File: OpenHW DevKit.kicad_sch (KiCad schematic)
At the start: 87 parts, among them Q1 MMBT3904, Q2 MMBT3904, Q3 MMBT3904, Q4 MMBT3904, SW1 SW_Push, SW2 SW_Push, U10 PI4ULS3V302XVEX, U13 PI4ULS3V302XVEX, U14 CORE-V-MCU, U15 PI4ULS3V302XVEX, U16 PI4ULS3V302XVEX, U17 PI4ULS3V302XVEX, U18 PI4ULS3V302XVEX, U19 PI4ULS3V302XVEX, U3 W25Q32JWZP, U4 PI6ULS5V9306WEX, U5 MAX6842DUKD0+T, U6 PI4ULS3V302XVEX, U7 PI4ULS3V302XVEX, U8 PI4ULS3V302XVEX, U9 PI4ULS3V302XVEX, X1 ECS-2520MVLC-100-CN

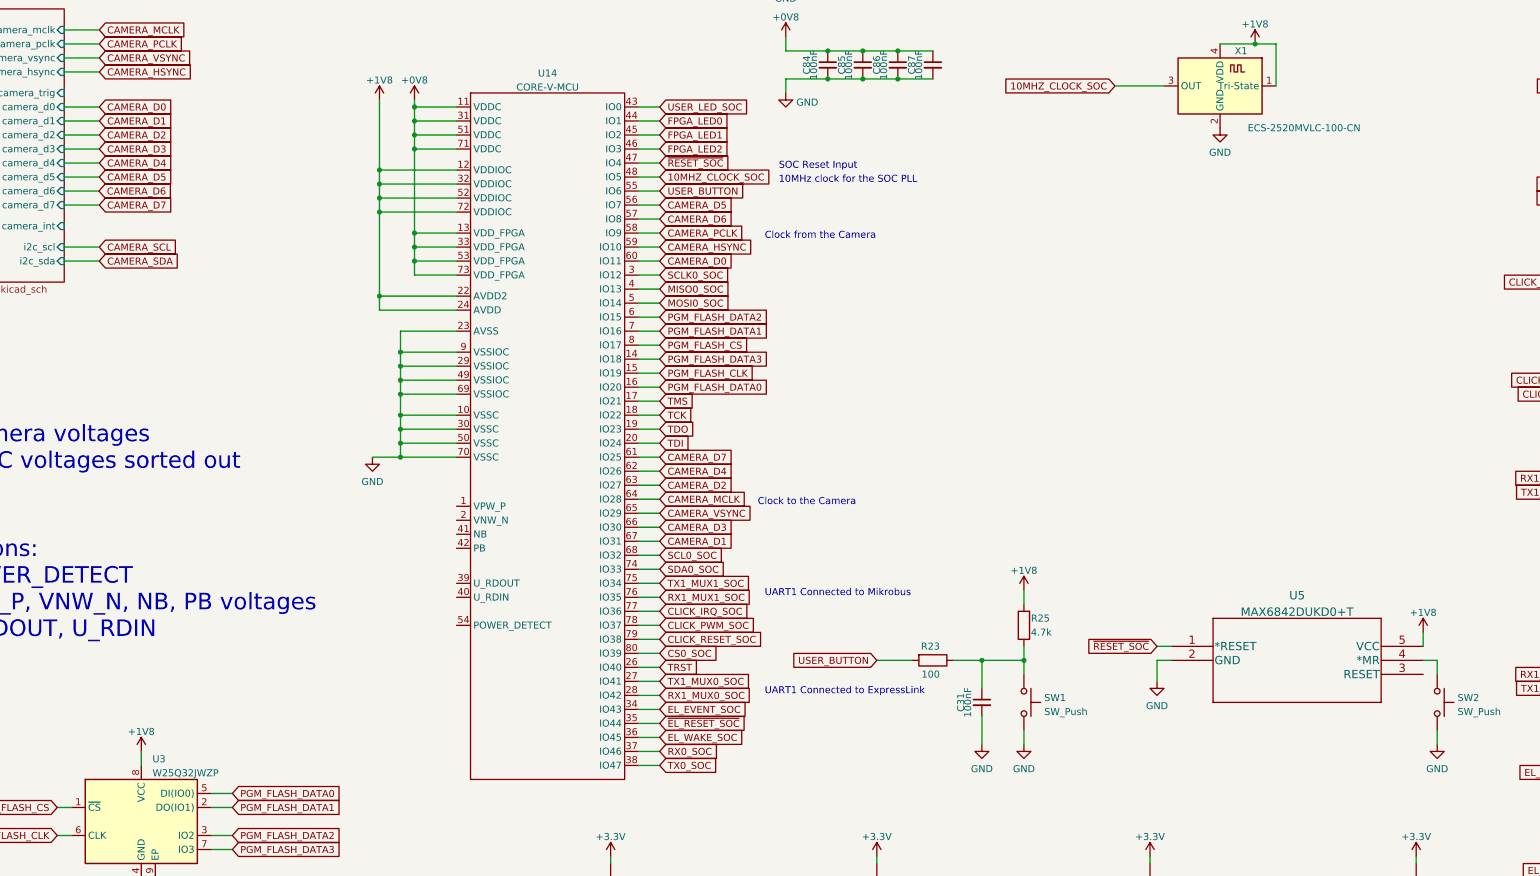
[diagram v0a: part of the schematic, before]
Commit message: revised pinout
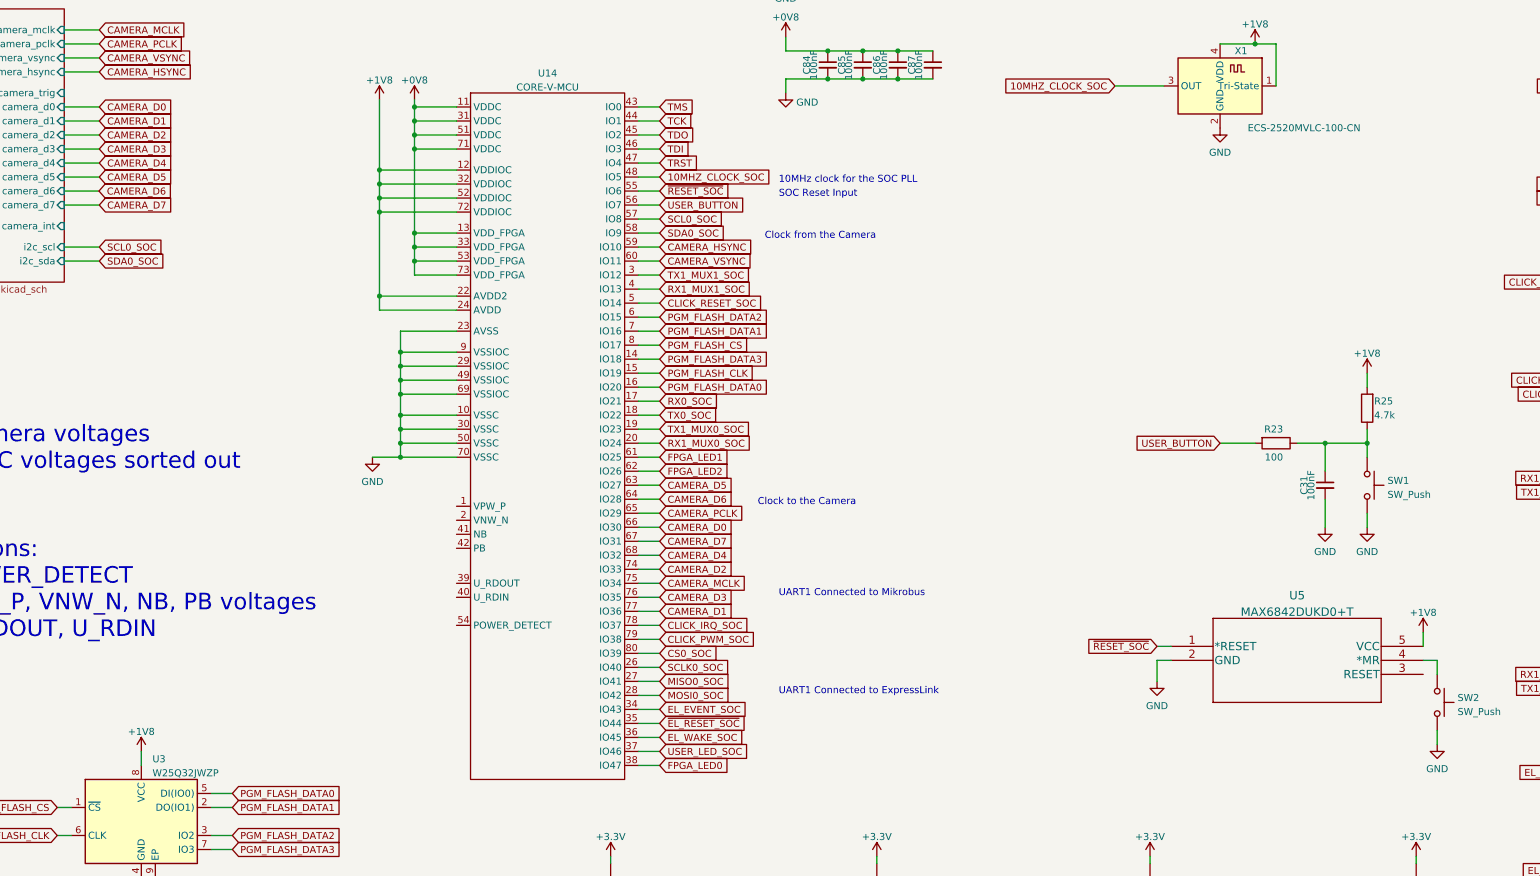
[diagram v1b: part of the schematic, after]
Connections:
- net CAMERA_D0: now also U14.66 (IO30); no longer U14.60 (IO11)
- net CAMERA_D1: now also U14.77 (IO36); no longer U14.67 (IO31)
- net CAMERA_D2: now also U14.74 (IO33); no longer U14.63 (IO27)
- net CAMERA_D3: now also U14.76 (IO35); no longer U14.66 (IO30)
- net CAMERA_D4: now also U14.68 (IO32); no longer U14.62 (IO26)
- net CAMERA_D5: now also U14.63 (IO27); no longer U14.56 (IO7)
- net CAMERA_D6: now also U14.64 (IO28); no longer U14.57 (IO8)
- net CAMERA_D7: now also U14.67 (IO31); no longer U14.61 (IO25)
- net CAMERA_MCLK: now also U14.75 (IO34); no longer U14.64 (IO28)
- net CAMERA_PCLK: now also U14.65 (IO29); no longer U14.58 (IO9)
- net CAMERA_VSYNC: now also U14.60 (IO11); no longer U14.65 (IO29)
- net CLICK_IRQ_SOC: now also U14.78 (IO37); no longer U14.77 (IO36)
- net CLICK_PWM_SOC: now also U14.79 (IO38); no longer U14.78 (IO37)
- net CLICK_RESET_SOC: now also U14.5 (IO14); no longer U14.79 (IO38)
- net FPGA_LED0: now also U14.38 (IO47); no longer U14.44 (IO1)
- net FPGA_LED1: now also U14.61 (IO25); no longer U14.45 (IO2)
- net FPGA_LED2: now also U14.62 (IO26); no longer U14.46 (IO3)
- net MISO0_SOC: now also U14.27 (IO41); no longer U14.4 (IO13)
- net MOSI0_SOC: now also U14.28 (IO42); no longer U14.5 (IO14)
- net RX0_SOC: now also U14.17 (IO21); no longer U14.37 (IO46)
- net RX1_MUX0_SOC: now also U14.20 (IO24); no longer U14.28 (IO42)
- net RX1_MUX1_SOC: now also U14.4 (IO13); no longer U14.76 (IO35)
- net SCL0_SOC: now also U14.57 (IO8); no longer U14.68 (IO32)
- net SCLK0_SOC: now also U14.26 (IO40); no longer U14.3 (IO12)
- net SDA0_SOC: now also U14.58 (IO9); no longer U14.74 (IO33)
- net TCK: now also U14.44 (IO1); no longer U14.18 (IO22)
- net TDI: now also U14.46 (IO3); no longer U14.20 (IO24)
- net TDO: now also U14.45 (IO2); no longer U14.19 (IO23)
- net TMS: now also U14.43 (IO0); no longer U14.17 (IO21)
- net TRST: now also U14.47 (IO4); no longer U14.26 (IO40)
- net TX0_SOC: now also U14.18 (IO22); no longer U14.38 (IO47)
- net TX1_MUX0_SOC: now also U14.19 (IO23); no longer U14.27 (IO41)
- net TX1_MUX1_SOC: now also U14.3 (IO12); no longer U14.75 (IO34)
- net USER_BUTTON: now also U14.56 (IO7); no longer U14.55 (IO6)
- net USER_LED_SOC: now also U14.37 (IO46); no longer U14.43 (IO0)
- net ~{RESET_SOC}: now also U14.55 (IO6); no longer U14.47 (IO4)
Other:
- moved on the sheet: C31, R23, R25, SW1

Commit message: Changed to KiCAD 7 and updated to final pinout.
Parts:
- removed C26, C27, C30, C38, C39, C42, C43, C44, C46, C47, C52, C53, C54, C56, C58, C60, C62, C64, C66, C67: 100nF, Capacitor_SMD:C_0603_1608Metric, symbol Device:C_Small
- removed U10, U13, U15, U16, U17, U18, U19, U6, U7, U8, U9: PI4ULS3V302XVEX, pi4uls3v302:PSON40P160X120X55-8N, symbol PI4ULS3V302XVEX:PI4ULS3V302XVEX
- removed U4: PI6ULS5V9306WEX, Package_SO:SOIC-8_3.9x4.9mm_P1.27mm, symbol PI6ULS5V9306:PI6ULS5V9306WEX
- added J10, J7, J8, J9: Conn_01x20, Connector_PinHeader_1.00mm:PinHeader_1x20_P1.00mm_Vertical, symbol Connector_Generic:Conn_01x20
- added JP2, JP6, JP7, JP8: SolderJumper_2_Bridged, Jumper:SolderJumper-2_P1.3mm_Bridged_RoundedPad1.0x1.5mm, symbol Jumper:SolderJumper_2_Bridged
- added SYM*1: ~, logos:devkits_qr, symbol OpenHW:Devkit_QR
- added TP1: TestPoint, TestPoint:TestPoint_Pad_D1.0mm, symbol Connector:TestPoint
- added U4: FXMA2102UMX, FXMA2102UMX:FXMA2102UMX, symbol FXMA2102UMX:FXMA2102UMX
- added U6, U7, U8, U9: NTB0104BQ,115, NTB0104:NXP_Semiconductors-SOT762-1-08_2019-0-MFG, symbol NTB0104:NTB0104BQ,115
- SW1, SW2: footprint Button_Switch_SMD:SW_Push_1P1T-SH_NO_CK_KMR2xxG -> Button:TS204225WT160SMTTR
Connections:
- net +0V8: now also U14.35 (VDD_FPGA), J10.11 (Pin_11), J10.13 (Pin_13), J7.11 (Pin_11), J7.13 (Pin_13), J8.13 (Pin_13), J8.15 (Pin_15), J9.11 (Pin_11), J9.13 (Pin_13); no longer U14.31 (VDDC)
- net +1V8: now also U14.23 (AVDD2), U14.25 (AVDD), U14.34 (VDDIOC), J10.12 (Pin_12), J7.12 (Pin_12), J8.14 (Pin_14), J8.3 (Pin_3), J8.5 (Pin_5), J9.12 (Pin_12), JP2.1 (A), JP8.1 (A), U4.8 (VCCB), U6.1 (VCC(A)), U6.8 (OE), U7.1 (VCC(A)), U7.8 (OE), U8.1 (VCC(A)), U8.8 (OE), U9.1 (VCC(A)), U9.8 (OE); no longer U14.22 (AVDD2), U14.24 (AVDD), U14.32 (VDDIOC)
- net +3V3: now also U6.14 (VCC(B)), U7.14 (VCC(B)), U8.14 (VCC(B)), U9.14 (VCC(B))
- net 10MHZ_CLOCK_SOC: now also J9.8 (Pin_8)
- net CAMERA_D0: now also U14.77 (IO30), J10.17 (Pin_17); no longer U14.66 (IO30)
- net CAMERA_D1: now also U14.67 (IO36), J10.7 (Pin_7); no longer U14.77 (IO36)
- net CAMERA_D2: now also U14.68 (IO33), J10.8 (Pin_8); no longer U14.74 (IO33)
- net CAMERA_D3: now also U14.64 (IO35), J10.4 (Pin_4); no longer U14.76 (IO35)
- net CAMERA_D4: now also U14.76 (IO32), J10.16 (Pin_16); no longer U14.68 (IO32)
- net CAMERA_D5: now also U14.36 (IO27), J8.16 (Pin_16); no longer U14.63 (IO27)
- net CAMERA_D6: now also U14.78 (IO28), J10.18 (Pin_18); no longer U14.64 (IO28)
- net CAMERA_D7: now also U14.74 (IO31), J10.14 (Pin_14); no longer U14.67 (IO31)
- net CAMERA_HSYNC: now also U14.20 (IO10), J7.20 (Pin_20); no longer U14.59 (IO10)
- net CAMERA_MCLK: now also U14.63 (IO34), J10.3 (Pin_3); no longer U14.75 (IO34)
- net CAMERA_PCLK: now also U14.66 (IO29), J10.6 (Pin_6); no longer U14.65 (IO29)
- net CAMERA_VSYNC: now also U14.3 (IO11), J7.3 (Pin_3); no longer U14.60 (IO11)
- net CLICK_CS: now also U7.10 (B4)
- net CLICK_INT: now also U8.12 (B2)
- net CLICK_IRQ_SOC: now also U14.38 (IO37), J8.18 (Pin_18), U8.3 (A2); no longer U14.78 (IO37)
- net CLICK_MISO: now also U7.12 (B2)
- net CLICK_MOSI: now also U7.13 (B1)
- net CLICK_PWM: now also U8.13 (B1)
- net CLICK_PWM_SOC: now also U14.80 (IO38), J10.20 (Pin_20), U8.2 (A1); no longer U14.79 (IO38)
- net CLICK_RESET_SOC: now also U14.16 (IO14), J7.16 (Pin_16), U6.5 (A4); no longer U14.5 (IO14)
- net CLICK_RST: now also U6.10 (B4)
- net CLICK_RX: now also U8.11 (B3)
- net CLICK_SCK: now also U7.11 (B3)
- net CLICK_TX: now also U8.10 (B4)
- net CONSOLE_RX: now also U9.13 (B1)
- net CONSOLE_TX: now also U9.12 (B2)
- net CS0_SOC: now also U14.30 (IO39), J8.10 (Pin_10), U7.5 (A4); no longer U14.80 (IO39)
- net EL_EVENT: now also U6.13 (B1)
- net EL_EVENT_SOC: now also U14.79 (IO43), J10.19 (Pin_19), U6.2 (A1); no longer U14.34 (IO43)
- net EL_RXD: now also U6.11 (B3)
- net EL_TXD: now also U6.12 (B2)
- net EL_WAKE: now also U9.11 (B3)
- net EL_WAKE_SOC: now also U14.39 (IO45), J8.19 (Pin_19), U9.4 (A3); no longer U14.36 (IO45)
- net FPGA_LED0: now also U14.62 (IO47), J10.2 (Pin_2); no longer U14.38 (IO47)
- net FPGA_LED1: now also U14.65 (IO25), J10.5 (Pin_5); no longer U14.61 (IO25)
- net FPGA_LED2: now also U14.75 (IO26), J10.15 (Pin_15); no longer U14.62 (IO26)
- net GND: now also U14.24 (AVSS), U14.31 (VSSIOC), U14.32 (VSSC), J10.10 (Pin_10), J10.9 (Pin_9), J7.10 (Pin_10), J7.9 (Pin_9), J8.11 (Pin_11), J8.12 (Pin_12), J8.4 (Pin_4), J9.10 (Pin_10), J9.9 (Pin_9), JP6.1 (A), JP7.1 (A), U4.4 (GND), U6.15 (GND), U6.7 (GND), U7.15 (GND), U7.7 (GND), U8.15 (GND), U8.7 (GND), U9.15 (GND), U9.7 (GND); no longer U14.23 (AVSS), U14.29 (VSSIOC), U14.30 (VSSC)
- net MISO0_SOC: now also U14.29 (IO41), J8.9 (Pin_9), U7.3 (A2); no longer U14.27 (IO41)
- net MOSI0_SOC: now also U14.40 (IO42), J8.20 (Pin_20), U7.2 (A1); no longer U14.28 (IO42)
- net PGM_FLASH_CLK: now also U14.6 (IO19), J7.6 (Pin_6); no longer U14.15 (IO19)
- net PGM_FLASH_CS: now also U14.56 (IO17), J9.16 (Pin_16); no longer U14.8 (IO17)
- net PGM_FLASH_DATA0: now also U14.14 (IO20), J7.14 (Pin_14); no longer U14.16 (IO20)
- net PGM_FLASH_DATA1: now also U14.15 (IO16), J7.15 (Pin_15); no longer U14.7 (IO16)
- net PGM_FLASH_DATA2: now also U14.7 (IO15), J7.7 (Pin_7); no longer U14.6 (IO15)
- net PGM_FLASH_DATA3: now also U14.5 (IO18), J7.5 (Pin_5); no longer U14.14 (IO18)
- net RX0_SOC: now also U14.60 (IO21), J9.20 (Pin_20), U9.3 (A2); no longer U14.17 (IO21)
- net RX1_MUX0_SOC: now also U14.58 (IO24), J9.18 (Pin_18), U6.3 (A2); no longer U14.20 (IO24)
- net RX1_MUX1_SOC: now also U14.8 (IO13), J7.8 (Pin_8), U8.4 (A3); no longer U14.4 (IO13)
- net SCL: now also U4.2 (A0)
- net SCL0_SOC: now also U14.18 (IO8), J7.18 (Pin_18), U4.7 (B0); no longer U14.57 (IO8)
- net SCLK0_SOC: now also U14.28 (IO40), J8.8 (Pin_8), U7.4 (A3); no longer U14.26 (IO40)
- net SDA: now also U4.3 (A1)
- net SDA0_SOC: now also U14.19 (IO9), J7.19 (Pin_19), U4.6 (B1); no longer U14.58 (IO9)
- net TCK: now also U14.46 (IO1), J9.6 (Pin_6); no longer U14.44 (IO1)
- net TDI: now also U14.43 (IO3), J9.3 (Pin_3); no longer U14.46 (IO3)
- net TDO: now also J9.5 (Pin_5)
- net TMS: now also U14.44 (IO0), J9.4 (Pin_4); no longer U14.43 (IO0)
- net TRST: now also J9.7 (Pin_7)
- net TX0_SOC: now also U14.59 (IO22), J9.19 (Pin_19), U9.2 (A1); no longer U14.18 (IO22)
- net TX1_MUX0_SOC: now also U14.57 (IO23), J9.17 (Pin_17), U6.4 (A3); no longer U14.19 (IO23)
- net TX1_MUX1_SOC: now also U14.4 (IO12), J7.4 (Pin_4), U8.5 (A4); no longer U14.3 (IO12)
- net USER_BUTTON: now also U14.17 (IO7), J7.17 (Pin_17); no longer U14.56 (IO7)
- net USER_LED_SOC: now also U14.61 (IO46), J10.1 (Pin_1); no longer U14.37 (IO46)
- net ~{EL_RESET_SOC}: now also U14.37 (IO44), J8.17 (Pin_17), U9.5 (A4); no longer U14.35 (IO44)
- net ~{EL_RESET}: now also U9.10 (B4)
- net ~{RESET_SOC}: now also J9.15 (Pin_15)
- net at C6.1, R18.1: now also U4.1 (VCCA), U4.5 (OE)
- net VPW_P: now reaches U14.1 (VPW_P)
- net VPW_P: now also J7.1 (Pin_1), JP2.2 (B)
- net VNW_N: now reaches U14.2 (VNW_N)
- net VNW_N: now also J7.2 (Pin_2), JP6.2 (B)
- net NB: now reaches U14.41 (NB)
- net NB: now also J9.1 (Pin_1), JP7.2 (B)
- net PB: now reaches U14.42 (PB)
- net PB: now also J9.2 (Pin_2), JP8.2 (B)
- net POWER_DETECT: now reaches U14.54 (POWER_DETECT)
- net POWER_DETECT: now also J9.14 (Pin_14), TP1.1
- no-connect marks 3 -> 2
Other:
- note added: "Note: Verify these connections. Do we need bypass capacitors?"
- note removed: "Questions: 1) POWER_DETECT 2) VPW_P, VNW_N, NB, PB voltages 3) U_RDOUT, U_RDIN"
- note removed: "TODO Fix Camera voltages Get SOC voltages sorted out"
- moved on the sheet: C28, C29, C31, C40, C41, C45, C48, C49, C50, C51, C55, C57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
